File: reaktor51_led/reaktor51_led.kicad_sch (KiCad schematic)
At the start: 4 parts, among them SW1 SW_SPST

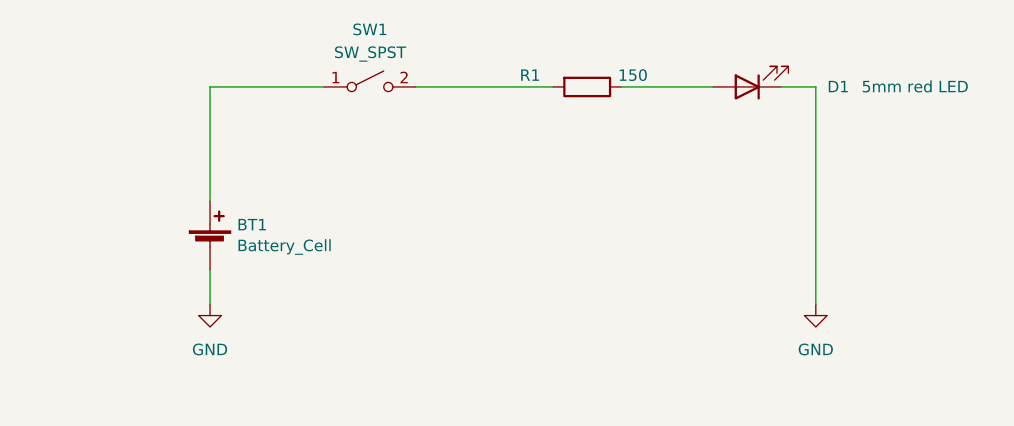
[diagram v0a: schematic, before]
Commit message: reaktor51_led rev1 rc2
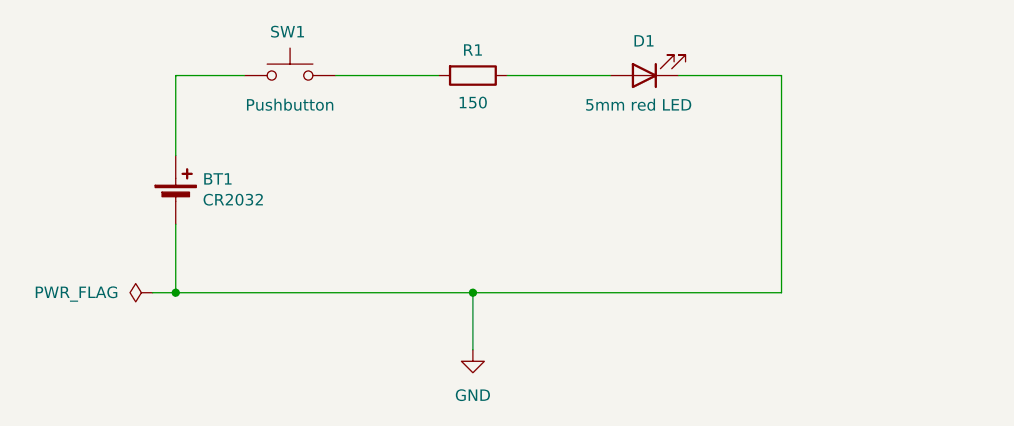
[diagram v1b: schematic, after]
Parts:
- BT1: value Battery_Cell -> CR2032
- SW1: value SW_SPST -> Pushbutton; symbol Switch:SW_SPST -> Switch:SW_Push
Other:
- title: (none) -> Reaktor51 LED
- moved on the sheet: BT1, D1, R1
